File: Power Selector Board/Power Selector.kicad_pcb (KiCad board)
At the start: 2 copper layers, 113.9 x 67.2 mm, 54 parts, among them J201 64900221122, J202 64900221122, J203 64900221122, J204 MSD-DB01M-12P, J205 1998865, J206 MSD-DB01F-12P_1, J301 64900221122, J302 1998865, J303 64900221122, J304 64900221122, J305 MSD-DB01M-12P, J306 MSD-DB01F-12P_1, K201 J115F11C24VDCSH.9, K202 G6SK-2G DC24, K203 J115F11C24VDCSH.9, K301 J115F11C24VDCSH.9, K302 G6SK-2G DC24, K303 J115F11C24VDCSH.9, U201 LMW78_24-0.3RL, U202 LMW78_24-0.3RL, U301 LMW78_24-0.3RL, U302 LMW78_24-0.3RL

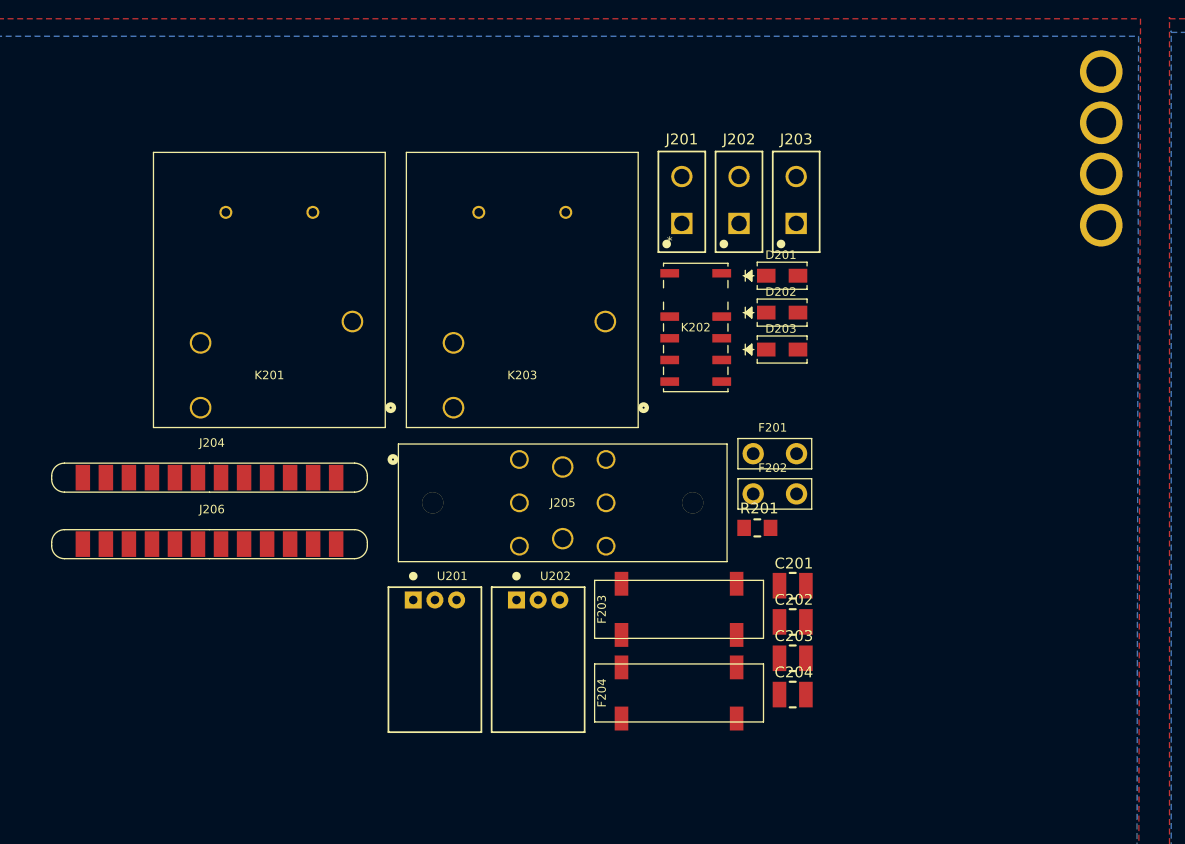
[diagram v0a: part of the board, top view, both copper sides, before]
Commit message: Routing PCB gauche. Prêt pour review 1.
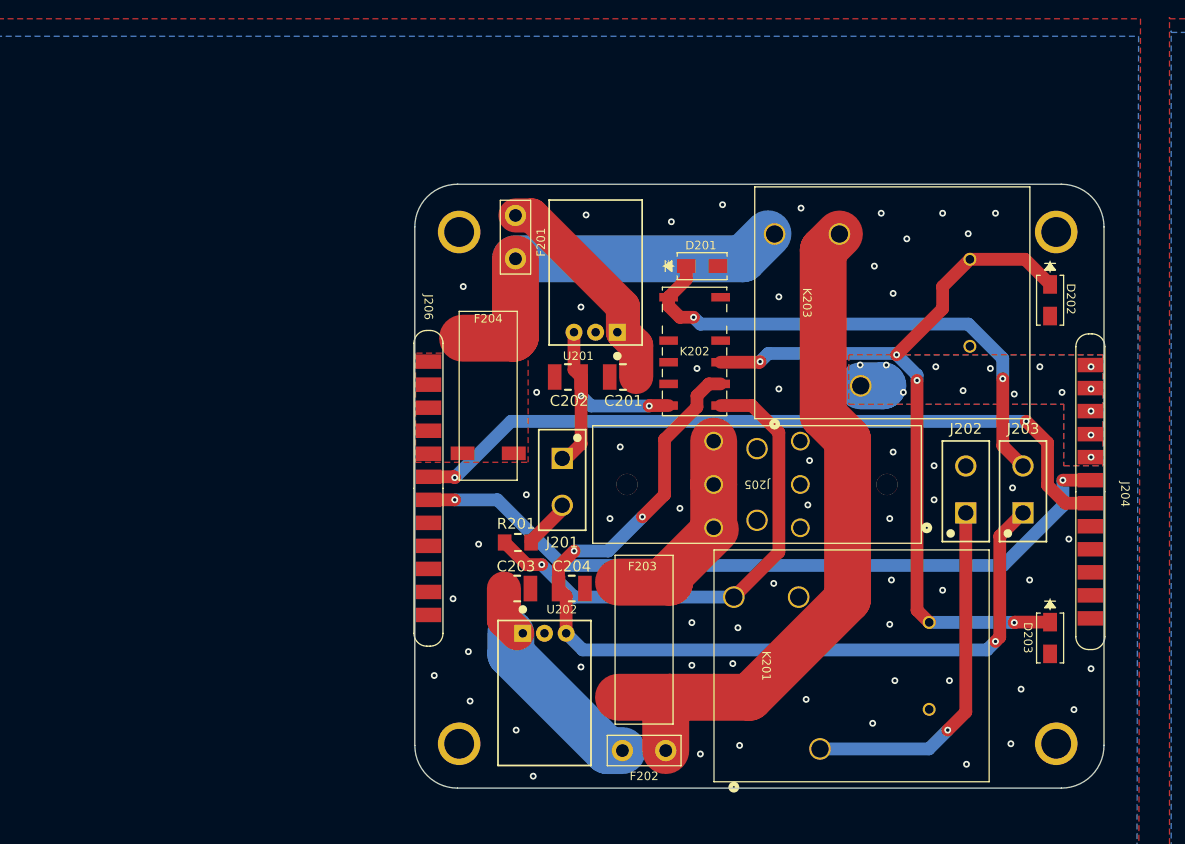
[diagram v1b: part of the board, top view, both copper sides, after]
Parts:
- moved J204 118.9 mm to (139.7, 85.8), turned to -90 degrees
- moved H4 96.8 mm to (65.7, 130.2)
- moved H3 75.6 mm to (65.7, 70.2)
- moved H2 73.0 mm to (135.7, 130.2)
- moved K201 66.3 mm to (97.9, 113.0), turned to -90 degrees
- moved D203 46.2 mm to (135.0, 117.8), turned to -90 degrees
- moved J206 45.8 mm to (62.1, 85.4), turned to -90 degrees
- moved J203 43.1 mm to (131.8, 100.3)
- moved J202 43.1 mm to (125.1, 100.3)
- moved K203 42.8 mm to (102.7, 70.4), turned to -90 degrees
- moved F204 41.4 mm to (69.1, 89.4), turned to -90 degrees
- moved F201 39.6 mm to (72.3, 70.8), turned to 90 degrees
- moved C202 39.0 mm to (76.9, 87.2)
- moved U201 36.6 mm to (81.7, 82.0), turned to 180 degrees
- moved J201 36.1 mm to (77.8, 99.6), turned to 180 degrees
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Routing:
- net 24V_Tether_G: track 0.00 -> 108.6 mm, vias 0 -> 3
- net /PCB_Gauche/Relay_Active: track 0.00 -> 93.7 mm, vias 0 -> 4
- net /PCB_Gauche/SDA: track 0.00 -> 87.3 mm, vias 0 -> 2
- net /PCB_Gauche/SCL: track 0.00 -> 86.7 mm, vias 0 -> 2
- net +Vin_Tether_G: track 0.00 -> 82.8 mm
- net Net-(D201-Pad1): track 0.00 -> 60.8 mm, vias 0 -> 2
- net Net-(K201-Pad1): track 0.00 -> 59.1 mm, vias 0 -> 1
- net Vin_Bat_G: track 0.00 -> 46.2 mm
- net Net-(J202-Pad1): track 0.00 -> 42.2 mm, vias 0 -> 1
- net 24V_Bat_G: track 0.00 -> 28.8 mm, vias 0 -> 2
- net Net-(U202-Vin): track 0.00 -> 26.1 mm
- net Net-(U201-Vin): track 0.00 -> 25.9 mm
- net Net-(F203-Pad2): track 0.00 -> 24.6 mm
- net Net-(J201-Pad2): track 0.00 -> 6.09 mm
- net +Vin_Drone_G: track 0.00 -> 2.62 mm, vias 0 -> 14
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- added copper zone on B.Cu, net +Vin_Drone_G
- added copper zone on F.Cu, net +Vin_Drone_G
- added copper zone on F.Cu, net Net-(F204-Pad2)
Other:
- board size 113.9 x 67.2 mm -> 213 x 70.8 mm
